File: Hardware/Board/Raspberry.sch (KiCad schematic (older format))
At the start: 7 parts, among them J6 Raspberry_Pi_2_3, U13 ESP-12F, U15 MOD-nRF8001

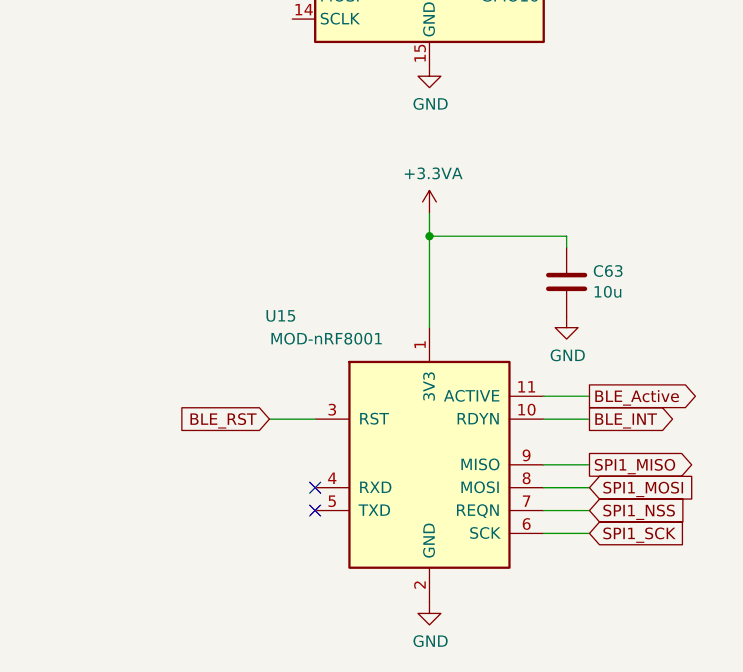
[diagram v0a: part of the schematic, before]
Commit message: Board to Board Verbindung eingefügt
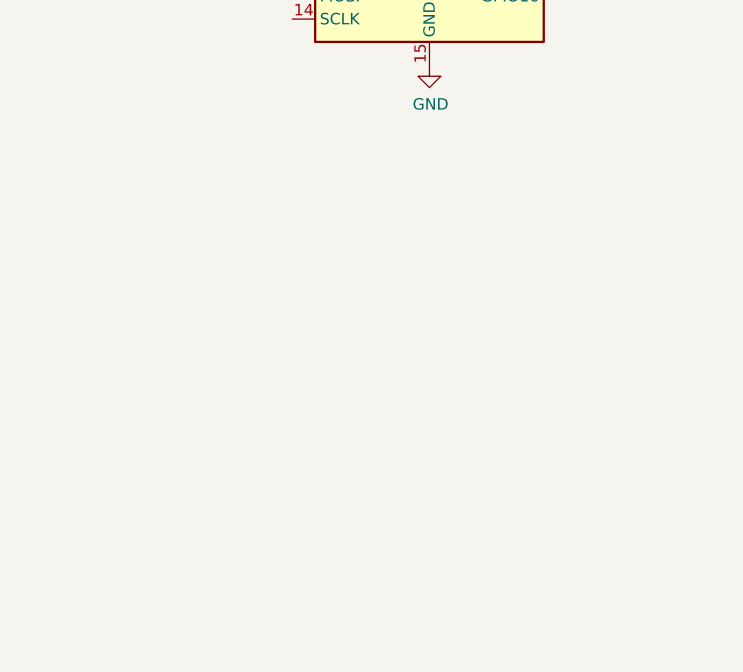
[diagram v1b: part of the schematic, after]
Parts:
- removed C63: 10u, Capacitor_SMD:C_1210_3225Metric, symbol Device:C
- removed U15: MOD-nRF8001, RF_Module:MOD-nRF8001, symbol RF_Bluetooth:MOD-nRF8001
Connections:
- no-connect marks 2 -> 0
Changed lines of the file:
@@
 EESchema Schematic File Version 4
 LIBS:Womo-cache
-EELAYER 29 0
+EELAYER 26 0
 EELAYER END
 $Descr A4 11693 8268
@@
 Wire Wire Line
 	7950 1350 8400 1350
-$Comp
-L RF_Bluetooth:MOD-nRF8001 U15
-U 1 1 5CDFE053
-P 7950 5200
-F 0 "U15" H 7300 5850 50  0000 C CNN
-F 1 "MOD-nRF8001" H 7500 5750 50  0000 C CNN
-F 2 "RF_Module:MOD-nRF8001" H 8000 5250 50  0001 C CNN
-F 3 "https://www.olimex.com/Products/Modules/RF/MOD-nRF8001/" H 8000 5200 50  0001 C CNN
-	1    7950 5200
-	1    0    0    -1
-$EndComp
-Text GLabel 8650 5300 2    50   Input ~ 0
-SPI1_MOSI
-Text GLabel 8650 5500 2    50   Input ~ 0
-SPI1_SCK
-Text GLabel 8650 5200 2    50   Output ~ 0
-SPI1_MISO
-$Comp
-L power:GND #PWR0249
-U 1 1 5CDFE14F
-P 7950 5800
-F 0 "#PWR0249" H 7950 5550 50  0001 C CNN
-F 1 "GND" H 7955 5627 50  0000 C CNN
-F 2 "" H 7950 5800 50  0001 C CNN
-F 3 "" H 7950 5800 50  0001 C CNN
-	1    7950 5800
-	1    0    0    -1
-$EndComp
-$Comp
-L Device:C C63
-U 1 1 5CDFE647
-P 8550 4400
-F 0 "C63" H 8665 4446 50  0000 L CNN
-F 1 "10u" H 8665 4355 50  0000 L CNN
-F 2 "Capacitor_SMD:C_1210_3225Metric" H 8588 4250 50  0001 C CNN
-F 3 "~" H 8550 4400 50  0001 C CNN
-	1    8550 4400
-	1    0    0    -1
-$EndComp
-$Comp
-L power:GND #PWR0250
-U 1 1 5CDFE64E
-P 8550 4550
-F 0 "#PWR0250" H 8550 4300 50  0001 C CNN
-F 1 "GND" H 8555 4377 50  0000 C CNN
-F 2 "" H 8550 4550 50  0001 C CNN
-F 3 "" H 8550 4550 50  0001 C CNN
-	1    8550 4550
-	1    0    0    -1
-$EndComp
-Wire Wire Line
-	8550 4250 8550 4200
-Wire Wire Line
-	8550 4200 7950 4200
-Wire Wire Line
-	7950 4200 7950 4600
-NoConn ~ 7450 5300
-NoConn ~ 7450 5400
-Text GLabel 8650 5400 2    50   Input ~ 0
-SPI1_NSS
-Text GLabel 8650 5000 2    50   Output ~ 0
-BLE_INT
-Text GLabel 8650 4900 2    50   Output ~ 0
-BLE_Active
-Text GLabel 7250 5000 0    50   Input ~ 0
-BLE_RST
-Wire Wire Line
-	7250 5000 7450 5000
-Wire Wire Line
-	8450 4900 8650 4900
-Wire Wire Line
-	8450 5000 8650 5000
-Wire Wire Line
-	8450 5200 8650 5200
-Wire Wire Line
-	8450 5300 8650 5300
-Wire Wire Line
-	8450 5400 8650 5400
-Wire Wire Line
-	8450 5500 8650 5500
 Text GLabel 8700 2450 2    50   Output ~ 0
 UART5_TX
@@
 $Comp
 L power:+3.3VA #PWR?
-U 1 1 5D4E449C
-P 7950 4100
-AR Path="/5C8BBC9A/5D4E449C" Ref="#PWR?"  Part="1"
-AR Path="/5E0C5EEA/5D4E449C" Ref="#PWR?"  Part="1"
-F 0 "#PWR?" H 7950 3950 50  0001 C CNN
-F 1 "+3.3VA" H 7965 4273 50  0000 C CNN
-F 2 "" H 7950 4100 50  0001 C CNN
-F 3 "" H 7950 4100 50  0001 C CNN
-	1    7950 4100
-	1    0    0    -1
-$EndComp
-Wire Wire Line
-	7950 4100 7950 4200
-Connection ~ 7950 4200
-$Comp
-L power:+3.3VA #PWR?
 U 1 1 5D4E6269
 P 7950 1250
 AR Path="/5C8BBC9A/5D4E6269" Ref="#PWR?"  Part="1"
 AR Path="/5E0C5EEA/5D4E6269" Ref="#PWR?"  Part="1"
-F 0 "#PWR?" H 7950 1100 50  0001 C CNN
+AR Path="/5C8BC88B/5D4E6269" Ref="#PWR0254"  Part="1"
+F 0 "#PWR0254" H 7950 1100 50  0001 C CNN
 F 1 "+3.3VA" H 7965 1423 50  0000 C CNN
 F 2 "" H 7950 1250 50  0001 C CNN
